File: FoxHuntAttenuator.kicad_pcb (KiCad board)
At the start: 2 copper layers, 34 parts, among them J1 Conn_Coaxial, J2 Conn_Coaxial, SW1 SW_SPST, SW2 SW_SPST, SW3 SW_SPST, SW4 SW_SPST, SW5 SW_SPST, SW6 SW_SPST, SW7 SW_SPST, SW8 SW_SPST

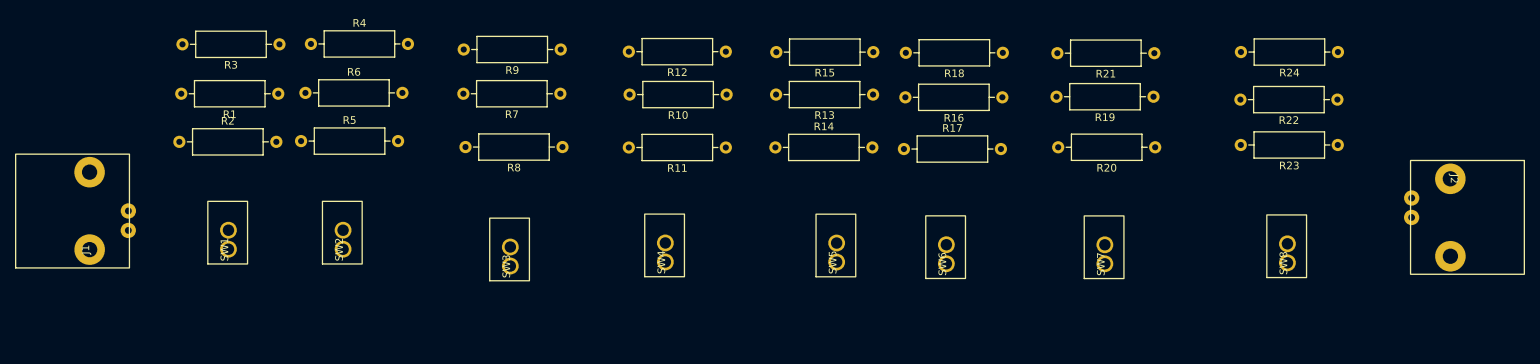
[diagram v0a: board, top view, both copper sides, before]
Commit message: working on pcb
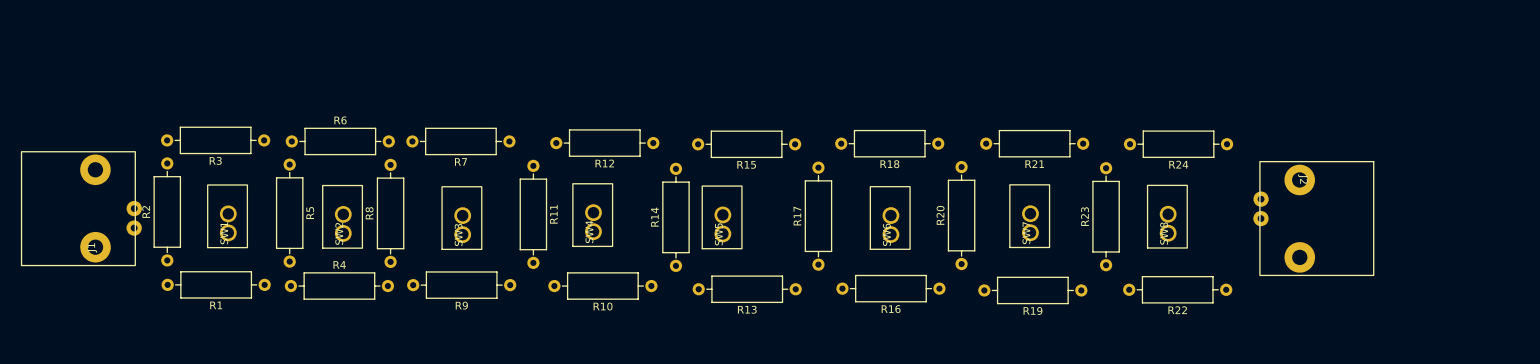
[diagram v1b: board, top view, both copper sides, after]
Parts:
- moved R23 34.2 mm to (210.9, 127.8), turned to 90 degrees
- moved R4 31.8 mm to (104.1, 130.5)
- moved R9 31.6 mm to (132.8, 130.4)
- moved R20 29.6 mm to (191.9, 127.7), turned to 90 degrees
- moved R22 28.8 mm to (226.6, 131.0)
- moved R13 27.4 mm to (170.2, 131.0)
- moved R19 27.1 mm to (207.6, 131.1)
- moved R8 27.1 mm to (117.2, 127.4), turned to 90 degrees
- moved R10 26.9 mm to (151.3, 130.5)
- moved R16 26.4 mm to (189.1, 130.9)
- moved R11 25.3 mm to (135.9, 114.8), turned to -90 degrees
- moved R1 25.1 mm to (100.7, 130.4)
- moved R14 20.3 mm to (154.6, 127.9), turned to 90 degrees
- moved J2 19.7 mm to (236.2, 116.7)
- moved R24 18.9 mm to (226.7, 112.0)
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
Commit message: pcb layout
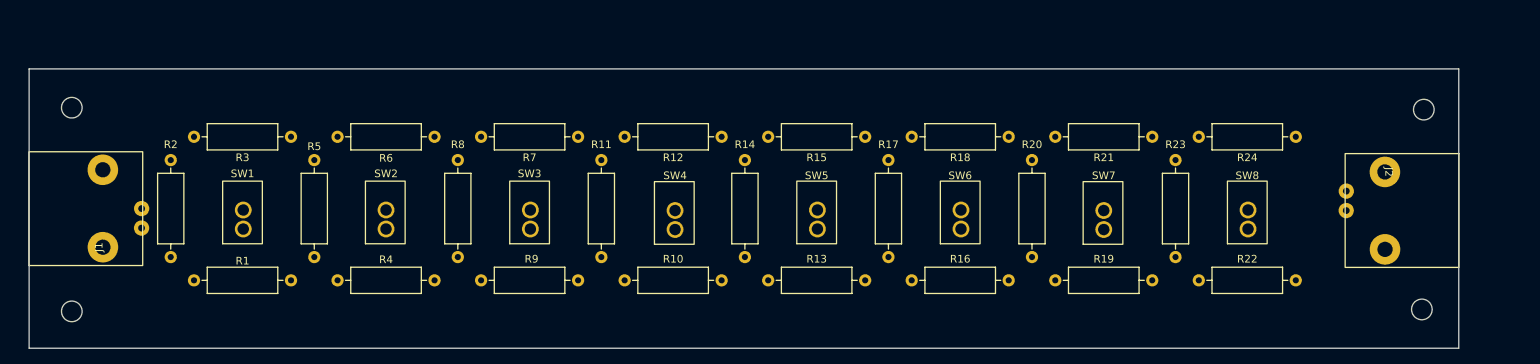
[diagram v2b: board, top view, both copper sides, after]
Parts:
- added H1: MountingHole, MountingHole:MountingHole_2.7mm_M2.5, F.Cu at (252.5, 107.4)
- added H2: MountingHole, MountingHole:MountingHole_2.7mm_M2.5, F.Cu at (252.2, 133.6)
- added H3: MountingHole, MountingHole:MountingHole_2.7mm_M2.5, F.Cu at (75.4, 133.9)
- added H4: MountingHole, MountingHole:MountingHole_2.7mm_M2.5, F.Cu at (75.4, 107.2)
- moved SW5 12.4 mm to (173.1, 123.1)
- moved J2 11.2 mm to (247.4, 115.6)
- moved SW4 10.7 mm to (154.4, 123.2)
- moved SW8 10.5 mm to (229.5, 123.1)
- moved SW7 9.61 mm to (210.6, 123.2)
- moved R19 9.38 mm to (216.9, 129.8)
- moved R18 9.27 mm to (198.1, 111.0)
- moved R20 9.26 mm to (201.2, 126.7)
- moved R10 9.23 mm to (160.5, 129.8)
- moved R15 9.23 mm to (179.3, 111.0)
- moved R17 9.22 mm to (182.4, 126.7)
- moved SW6 9.20 mm to (191.9, 123.1)
- moved R22 9.20 mm to (235.7, 129.8)
- moved R13 9.17 mm to (179.3, 129.8)
- moved R23 9.16 mm to (220.0, 126.7)
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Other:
- board outline added: 187.2 x 36.6 mm
